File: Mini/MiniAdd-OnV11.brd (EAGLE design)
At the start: 28.1 x 17.6 mm, 10 parts, among them X1 1501_03

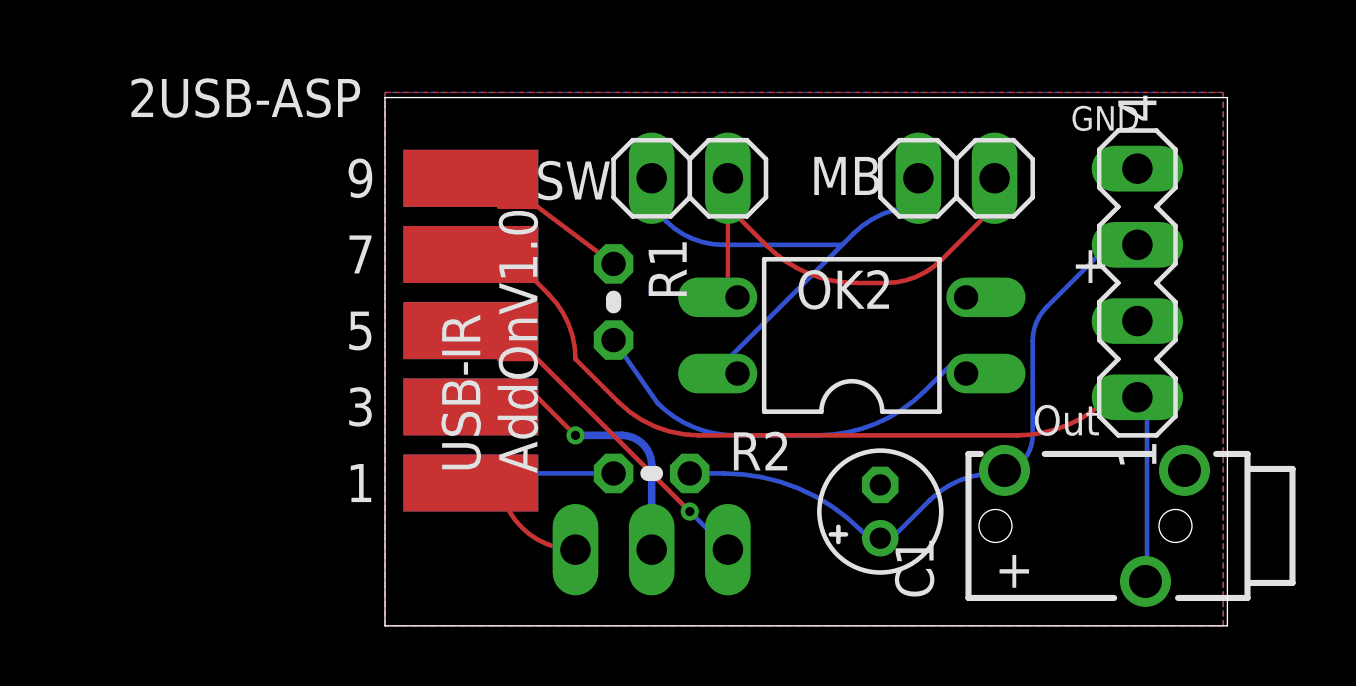
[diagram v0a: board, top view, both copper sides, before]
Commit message: Final Layout
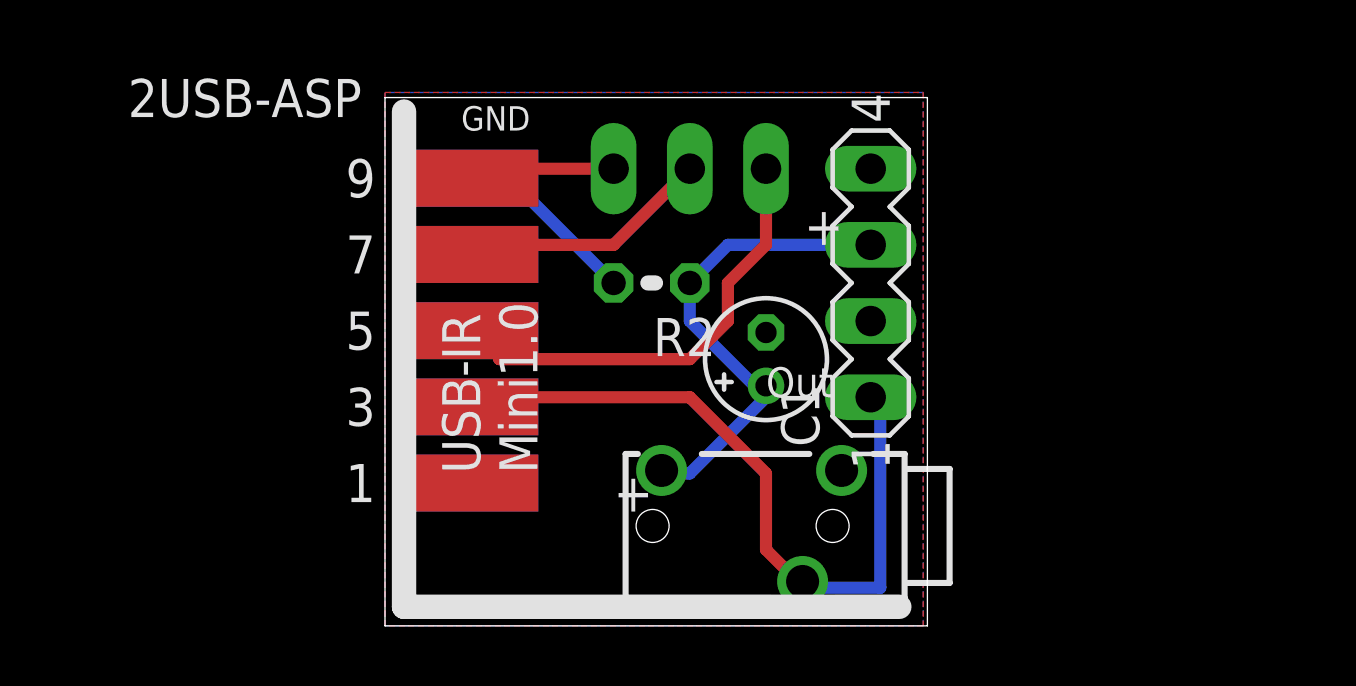
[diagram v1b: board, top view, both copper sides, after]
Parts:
- removed MB, SW: (no value), pinhead:1X02
- removed OK2: PC817, optocoupler:DIL04
- removed R1: 100, rcl:0204V
- moved FREI 12.8 mm to (10.2, 15.2), turned to 180 degrees
- moved X1 11.4 mm to (14.9, 3.33)
- moved SV1 8.89 mm to (16.2, 11.4)
- moved C1 6.35 mm to (12.7, 8.89)
- moved R2 6.35 mm to (8.89, 11.4)
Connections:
- removed net N$2: OK2.1, R1.2
- removed net N$3: MB.2, OK2.4, SW.1
- removed net N$4: MB.1, OK2.3, SW.2
- net GND: now also 2USB-ASP.P$2; no longer 2USB-ASP.P$10, OK2.2
- net MISO: now also 2USB-ASP.P$1; no longer 2USB-ASP.P$9, R1.1
- net MOSI: now also 2USB-ASP.P$9, FREI.1; no longer 2USB-ASP.P$1, FREI.3
- net NC: now also 2USB-ASP.P$7; no longer 2USB-ASP.P$3
- net RST: now also FREI.3; no longer FREI.1
- net SCK: now also 2USB-ASP.P$3; no longer 2USB-ASP.P$7
- net VCC: now also 2USB-ASP.P$10; no longer 2USB-ASP.P$2
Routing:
- net N$3: track 17.4 -> 0.00 mm
- net N$4: track 15.6 -> 0.00 mm
- net N$2: track 14.1 -> 0.00 mm
- net SCK: track 32.4 -> 24.9 mm
- net MISO: track 6.72 -> 0.00 mm
- net N$1: track 22.4 -> 17.4 mm
- net RST: track 12.5 -> 16.0 mm, vias 1 -> 0
- net VCC: track 4.81 -> 6.39 mm
- net NC: track 9.83 -> 8.40 mm, vias 1 -> 0
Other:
- board size 28.1 x 17.6 mm -> 18.1 x 17.6 mm
- board text added: "USB-IR Mini1.0"
- board text removed: "USB-IR AddOnV1.0"
